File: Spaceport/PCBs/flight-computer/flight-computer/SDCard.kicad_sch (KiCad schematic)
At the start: 0 parts

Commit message: something broke and git does not let me change branches
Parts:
- added J6: Micro_SD_Card, Connector_Card:microSD_HC_Molex_47219-2001, symbol Connector:Micro_SD_Card
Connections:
- new net +3V3: J6.4 (VDD)
- new net GND: J6.6 (VSS), J6.9 (SHIELD)
- new net SDMMC1_CK: J6.5 (CLK)
- new net SDMMC1_CMD: J6.3 (CMD)
- new net SDMMC1_D0: J6.7 (DAT0)
- new net SDMMC1_D1: J6.8 (DAT1)
- new net SDMMC1_D2: J6.1 (DAT2)
- new net SDMMC1_D3: J6.2 (DAT3/CD)

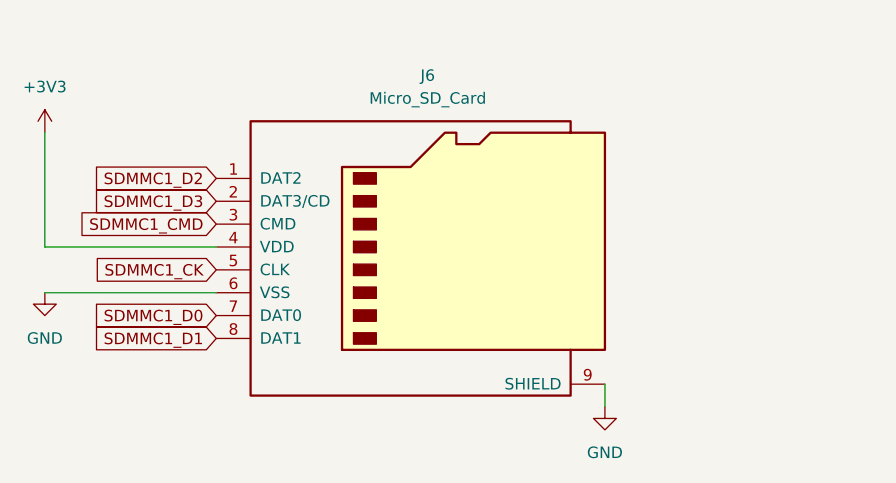
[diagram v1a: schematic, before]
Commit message: push for schematic review
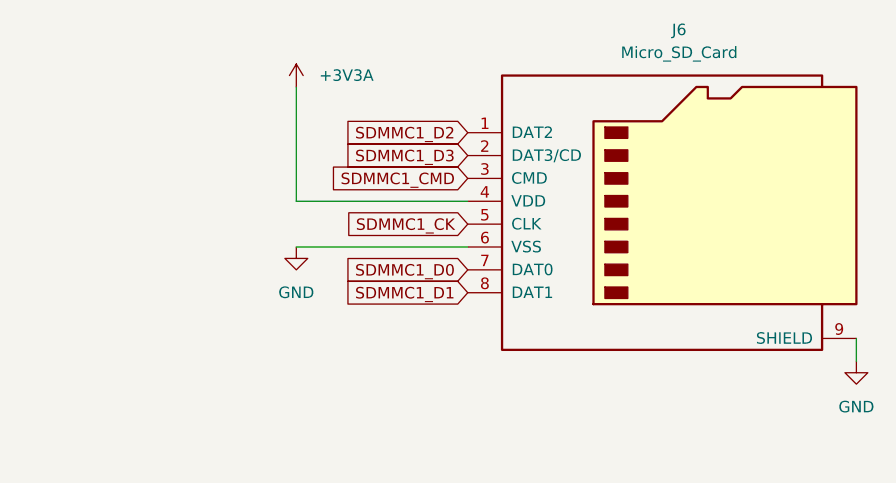
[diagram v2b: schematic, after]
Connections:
- net +3V3 renamed +3V3A
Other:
- moved on the sheet: J6
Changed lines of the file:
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@@
 	(wire
 		(pts
-			(xy 144.78 120.65) (xy 144.78 123.19)
+			(xy 110.49 87.63) (xy 110.49 100.33)
 		)
 		(stroke
@@
 	(wire
 		(pts
-			(xy 82.55 92.71) (xy 82.55 105.41)
+			(xy 110.49 105.41) (xy 129.54 105.41)
 		)
 		(stroke
@@
 	(wire
 		(pts
-			(xy 82.55 110.49) (xy 101.6 110.49)
+			(xy 129.54 100.33) (xy 110.49 100.33)
 		)
 		(stroke
@@
 	(wire
 		(pts
-			(xy 101.6 105.41) (xy 82.55 105.41)
+			(xy 172.72 115.57) (xy 172.72 118.11)
 		)
 		(stroke
@@
 		)
 	)
+	(global_label "SDMMC1_D3"
+		(shape input)
+		(at 129.54 95.25 180)
+		(fields_autoplaced yes)
+		(effects
+			(font
+				(size 1.27 1.27)
+			)
+			(justify right)
+		)
+		(property "Intersheetrefs" "${INTERSHEET_REFS}"
+			(at 115.2459 95.25 0)
+			(effects
+				(font
+					(size 1.27 1.27)
+				)
+				(justify right)
+				(hide yes)
+			)
+		)
+	)
+	(global_label "SDMMC1_CK"
+		(shape input)
+		(at 129.54 102.87 180)
+		(fields_autoplaced yes)
+		(effects
+			(font
+				(size 1.27 1.27)
+			)
+			(justify right)
+		)
+		(property "Intersheetrefs" "${INTERSHEET_REFS}"
+			(at 115.1854 102.87 0)
+			(effects
+				(font
+					(size 1.27 1.27)
+				)
+				(justify right)
+				(hide yes)
+			)
+		)
+	)
+	(global_label "SDMMC1_D2"
+		(shape input)
+		(at 129.54 92.71 180)
+		(fields_autoplaced yes)
+		(effects
+			(font
+				(size 1.27 1.27)
+			)
+			(justify right)
+		)
+		(property "Intersheetrefs" "${INTERSHEET_REFS}"
+			(at 115.2459 92.71 0)
+			(effects
+				(font
+					(size 1.27 1.27)
+				)
+				(justify right)
+				(hide yes)
+			)
+		)
+	)
+	(global_label "SDMMC1_D0"
+		(shape input)
+		(at 129.54 107.95 180)
+		(fields_autoplaced yes)
+		(effects
+			(font
+				(size 1.27 1.27)
+			)
+			(justify right)
+		)
+		(property "Intersheetrefs" "${INTERSHEET_REFS}"
+			(at 115.2459 107.95 0)
+			(effects
+				(font
+					(size 1.27 1.27)
+				)
+				(justify right)
+				(hide yes)
+			)
+		)
+	)
+	(global_label "SDMMC1_CMD"
+		(shape input)
+		(at 129.54 97.79 180)
+		(fields_autoplaced yes)
+		(effects
+			(font
+				(size 1.27 1.27)
+			)
+			(justify right)
+		)
+		(property "Intersheetrefs" "${INTERSHEET_REFS}"
+			(at 113.734 97.79 0)
+			(effects
+				(font
+					(size 1.27 1.27)
+				)
+				(justify right)
+				(hide yes)
+			)
+		)
+	)
 	(global_label "SDMMC1_D1"
 		(shape input)
-		(at 101.6 115.57 180)
-		(fields_autoplaced yes)
-		(effects
-			(font
-				(size 1.27 1.27)
-			)
-			(justify right)
-		)
-		(property "Intersheetrefs" "${INTERSHEET_REFS}"
-			(at 87.3059 115.57 0)
-			(effects
-				(font
-					(size 1.27 1.27)
-				)
-				(justify right)
-				(hide yes)
-			)
-		)
-	)
-	(global_label "SDMMC1_D0"
-		(shape input)
-		(at 101.6 113.03 180)
-		(fields_autoplaced yes)
-		(effects
-			(font
-				(size 1.27 1.27)
-			)
-			(justify right)
-		)
-		(property "Intersheetrefs" "${INTERSHEET_REFS}"
-			(at 87.3059 113.03 0)
-			(effects
-				(font
-					(size 1.27 1.27)
-				)
-				(justify right)
-				(hide yes)
-			)
-		)
-	)
-	(global_label "SDMMC1_CMD"
-		(shape input)
-		(at 101.6 102.87 180)
-		(fields_autoplaced yes)
-		(effects
-			(font
-				(size 1.27 1.27)
-			)
-			(justify right)
-		)
-		(property "Intersheetrefs" "${INTERSHEET_REFS}"
-			(at 85.794 102.87 0)
-			(effects
-				(font
-					(size 1.27 1.27)
-				)
-				(justify right)
-				(hide yes)
-			)
-		)
-	)
-	(global_label "SDMMC1_D3"
-		(shape input)
-		(at 101.6 100.33 180)
-		(fields_autoplaced yes)
-		(effects
-			(font
-				(size 1.27 1.27)
-			)
-			(justify right)
-		)
-		(property "Intersheetrefs" "${INTERSHEET_REFS}"
-			(at 87.3059 100.33 0)
-			(effects
-				(font
-					(size 1.27 1.27)
-				)
-				(justify right)
-				(hide yes)
-			)
-		)
-	)
-	(global_label "SDMMC1_D2"
-		(shape input)
-		(at 101.6 97.79 180)
-		(fields_autoplaced yes)
-		(effects
-			(font
-				(size 1.27 1.27)
-			)
-			(justify right)
-		)
-		(property "Intersheetrefs" "${INTERSHEET_REFS}"
-			(at 87.3059 97.79 0)
-			(effects
-				(font
-					(size 1.27 1.27)
-				)
-				(justify right)
-				(hide yes)
-			)
-		)
-	)
-	(global_label "SDMMC1_CK"
-		(shape input)
-		(at 101.6 107.95 180)
-		(fields_autoplaced yes)
-		(effects
-			(font
-				(size 1.27 1.27)
-			)
-			(justify right)
-		)
-		(property "Intersheetrefs" "${INTERSHEET_REFS}"
-			(at 87.2454 107.95 0)
+		(at 129.54 110.49 180)
+		(fields_autoplaced yes)
+		(effects
+			(font
+				(size 1.27 1.27)
+			)
+			(justify right)
+		)
+		(property "Intersheetrefs" "${INTERSHEET_REFS}"
+			(at 115.2459 110.49 0)
 			(effects
 				(font
@@
 	(symbol
 		(lib_id "power:GND")
-		(at 144.78 123.19 0)
+		(at 172.72 118.11 0)
 		(unit 1)
 		(exclude_from_sim no)
@@
 		(fields_autoplaced yes)
 		(property "Reference" "#PWR019"
-			(at 144.78 129.54 0)
+			(at 172.72 124.46 0)
 			(effects
 				(font
@@
 		)
 		(property "Value" "GND"
-			(at 144.78 128.27 0)
+			(at 172.72 123.19 0)
 			(effects
 				(font
@@
 		)
 		(property "Footprint" ""
-			(at 144.78 123.19 0)
+			(at 172.72 118.11 0)
 			(effects
 				(font
@@
 		)
 		(property "Datasheet" ""
-			(at 144.78 123.19 0)
+			(at 172.72 118.11 0)
 			(effects
 				(font
@@
 		)
 		(property "Description" "Power symbol creates a global label with name \"GND\" , ground"
-			(at 144.78 123.19 0)
+			(at 172.72 118.11 0)
 			(effects
 				(font
@@
 		)
 		(instances
-			(project ""
+			(project "flight-computer"
 				(path "/b419aaf0-5349-42bc-a414-d94cafbe45e9/cf915fab-afce-462a-afc9-9be0ef6a3002"
 					(reference "#PWR019")
@@
 	(symbol
 		(lib_id "power:GND")
-		(at 82.55 110.49 0)
+		(at 110.49 105.41 0)
 		(unit 1)
 		(exclude_from_sim no)
@@
 		(fields_autoplaced yes)
 		(property "Reference" "#PWR021"
-			(at 82.55 116.84 0)
+			(at 110.49 111.76 0)
 			(effects
 				(font
@@
 		)
 		(property "Value" "GND"
-			(at 82.55 115.57 0)
+			(at 110.49 110.49 0)
 			(effects
 				(font
@@
 		)
 		(property "Footprint" ""
-			(at 82.55 110.49 0)
+			(at 110.49 105.41 0)
 			(effects
 				(font
@@
 		)
 		(property "Datasheet" ""
-			(at 82.55 110.49 0)
+			(at 110.49 105.41 0)
 			(effects
 				(font
@@
 		)
 		(property "Description" "Power symbol creates a global label with name \"GND\" , ground"
-			(at 82.55 110.49 0)
+			(at 110.49 105.41 0)
 			(effects
 				(font
@@
 	(symbol
 		(lib_id "Connector:Micro_SD_Card")
-		(at 124.46 105.41 0)
+		(at 152.4 100.33 0)
 		(unit 1)
 		(exclude_from_sim no)
@@
 		(fields_autoplaced yes)
 		(property "Reference" "J6"
-			(at 125.095 86.36 0)
+			(at 153.035 81.28 0)
 			(effects
 				(font
@@
 		)
 		(property "Value" "Micro_SD_Card"
-			(at 125.095 88.9 0)
+			(at 153.035 83.82 0)
 			(effects
 				(font
@@
 		)
 		(property "Footprint" "Connector_Card:microSD_HC_Molex_47219-2001"
-			(at 153.67 97.79 0)
+			(at 181.61 92.71 0)
 			(effects
 				(font
@@
 		)
 		(property "Datasheet" "https://www.we-online.com/components/products/datasheet/693072010801.pdf"
-			(at 124.46 105.41 0)
+			(at 152.4 100.33 0)
 			(effects
 				(font
@@
 		)
 		(property "Description" "Micro SD Card Socket"
-			(at 124.46 105.41 0)
+			(at 152.4 100.33 0)
 			(effects
 				(font
@@
 		)
 		(instances
-			(project ""
+			(project "flight-computer"
 				(path "/b419aaf0-5349-42bc-a414-d94cafbe45e9/cf915fab-afce-462a-afc9-9be0ef6a3002"
 					(reference "J6")
@@
 	(symbol
 		(lib_id "power:+3V3")
-		(at 82.55 92.71 0)
+		(at 110.49 87.63 0)
 		(unit 1)
 		(exclude_from_sim no)
@@
 		(fields_autoplaced yes)
 		(property "Reference" "#PWR020"
-			(at 82.55 96.52 0)
-			(effects
-				(font
-					(size 1.27 1.27)
-				)
-				(hide yes)
-			)
-		)
-		(property "Value" "+3V3"
-			(at 82.55 87.63 0)
-			(effects
-				(font
-					(size 1.27 1.27)
-				)
+			(at 110.49 91.44 0)
+			(effects
+				(font
+					(size 1.27 1.27)
+				)
+				(hide yes)
+			)
+		)
+		(property "Value" "+3V3A"
+			(at 113.03 86.3599 0)
+			(effects
+				(font
+					(size 1.27 1.27)
+				)
+				(justify left)
 			)
 		)
 		(property "Footprint" ""
-			(at 82.55 92.71 0)
+			(at 110.49 87.63 0)
 			(effects
 				(font
@@
 		)
 		(property "Datasheet" ""
-			(at 82.55 92.71 0)
+			(at 110.49 87.63 0)
 			(effects
 				(font
@@
 		)
 		(property "Description" "Power symbol creates a global label with name \"+3V3\""
-			(at 82.55 92.71 0)
+			(at 110.49 87.63 0)
 			(effects
 				(font
@@
 		)
 		(instances
-			(project ""
+			(project "flight-computer"
 				(path "/b419aaf0-5349-42bc-a414-d94cafbe45e9/cf915fab-afce-462a-afc9-9be0ef6a3002"
 					(reference "#PWR020")
